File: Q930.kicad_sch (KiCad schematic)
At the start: 15 parts, among them J1 7Pin, U1 MW-R-WX, U2 DRV5032FDDMRR, U3 SHT40I-AD1B-R2, U4 TPL5010DDCR

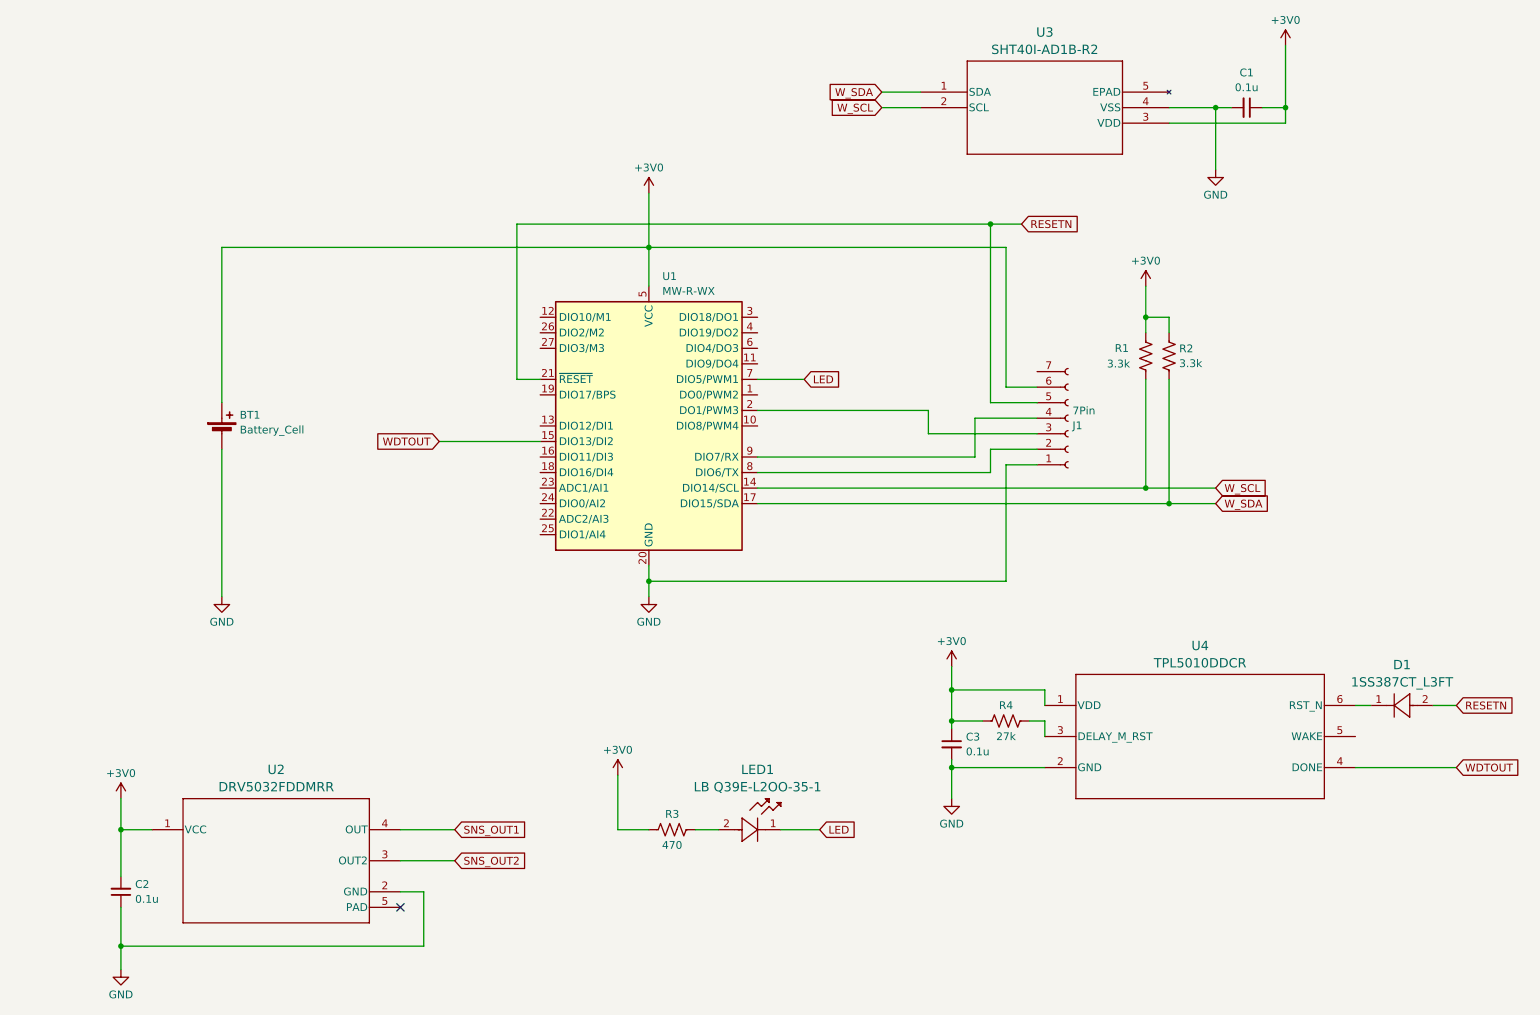
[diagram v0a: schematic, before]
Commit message: 途中
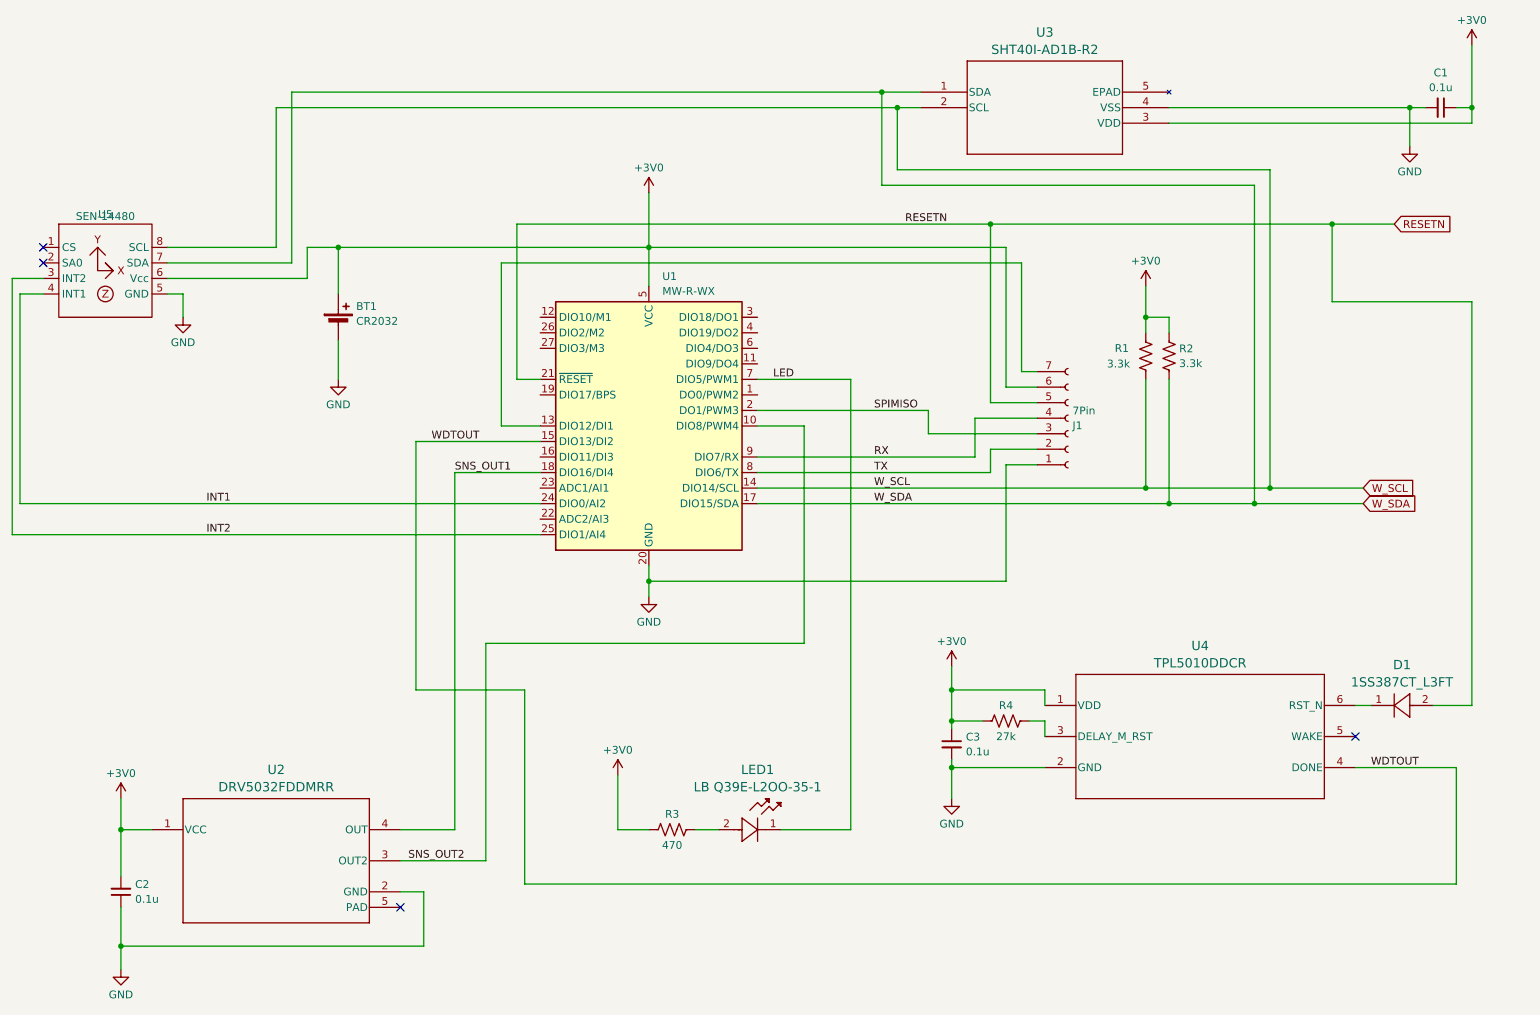
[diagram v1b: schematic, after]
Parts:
- added U5: SEN-14480, q930:SEN-14480, symbol q930:SEN-14480
- BT1: value Battery_Cell -> CR2032
- J1: footprint (none) -> Connector_PinSocket_2.54mm:PinSocket_1x07_P2.54mm_Vertical_SMD_Pin1Left
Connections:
- net +3V0: now also U5.6 (Vcc)
- net GND: now also U5.5 (GND)
- net SNS_OUT1: now also U1.18 (DIO16/DI4)
- net SNS_OUT2: now also U1.10 (DIO8/PWM4)
- net W_SCL: now also U5.8 (SCL)
- net W_SDA: now also U5.7 (SDA)
- net TX: now reaches J1.2 (Pin_2), U1.8 (DIO6/TX)
- net SPIMISO: now reaches J1.3 (Pin_3), U1.2 (DO1/PWM3)
- net RX: now reaches J1.4 (Pin_4), U1.9 (DIO7/RX)
- net at J1.7 (Pin_7): now also U1.13 (DIO12/DI1)
- net INT1: now reaches U1.24 (DIO0/AI2)
- net INT1: now also U5.4 (INT1)
- net INT2: now reaches U1.25 (DIO1/AI4)
- net INT2: now also U5.3 (INT2)
- no-connect marks 1 -> 4
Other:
- moved on the sheet: BT1, C1
